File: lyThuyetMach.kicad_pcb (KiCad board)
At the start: 2 copper layers, 48 x 79 mm, 34 parts, among them J1 USB_C_Receptacle_PowerOnly_6P, J2 Voltage_Booster, J4 Out_LED, Q1 BC547, Q2 BC547, Q3 BC547, Q4 BC547, Q5 BC547, Q6 BC547, Q7 TIP122, SW1 SW_SPDT, SW2 SW_SPDT

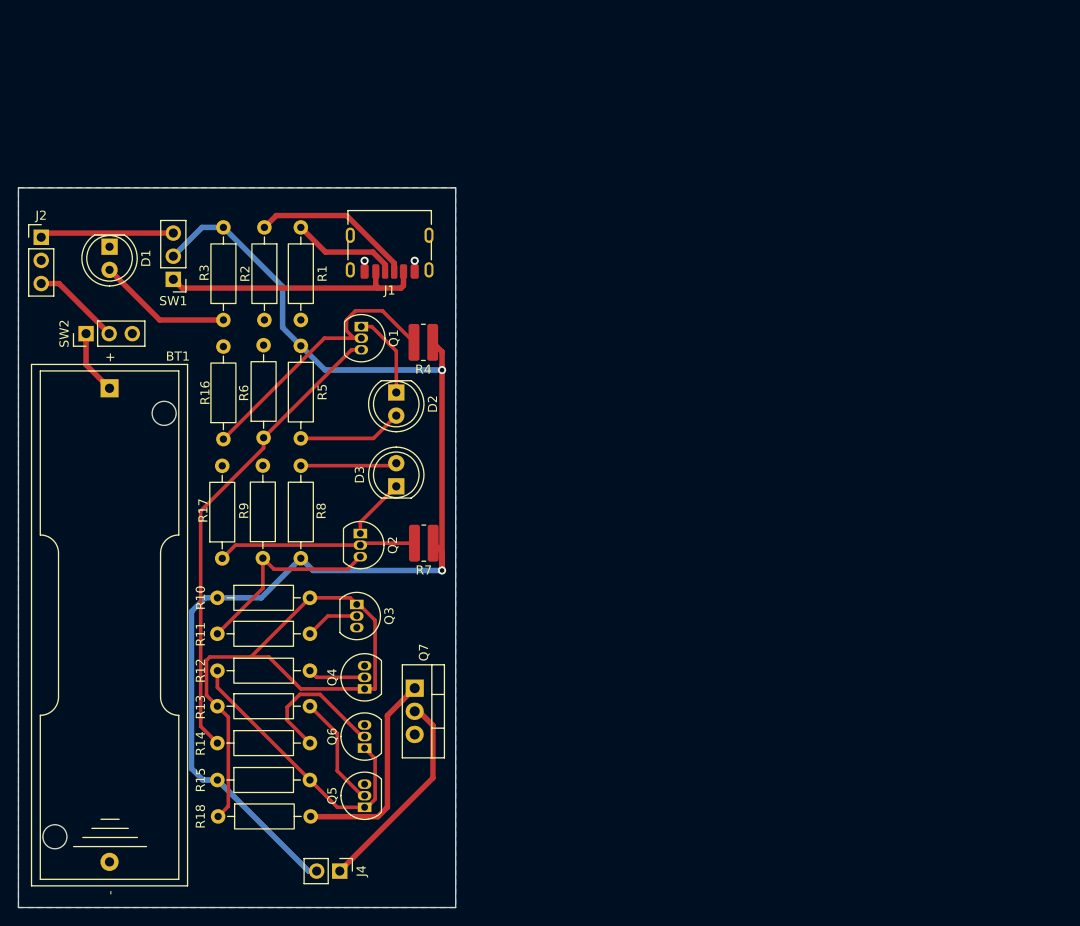
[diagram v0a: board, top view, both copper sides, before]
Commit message: Add files via upload
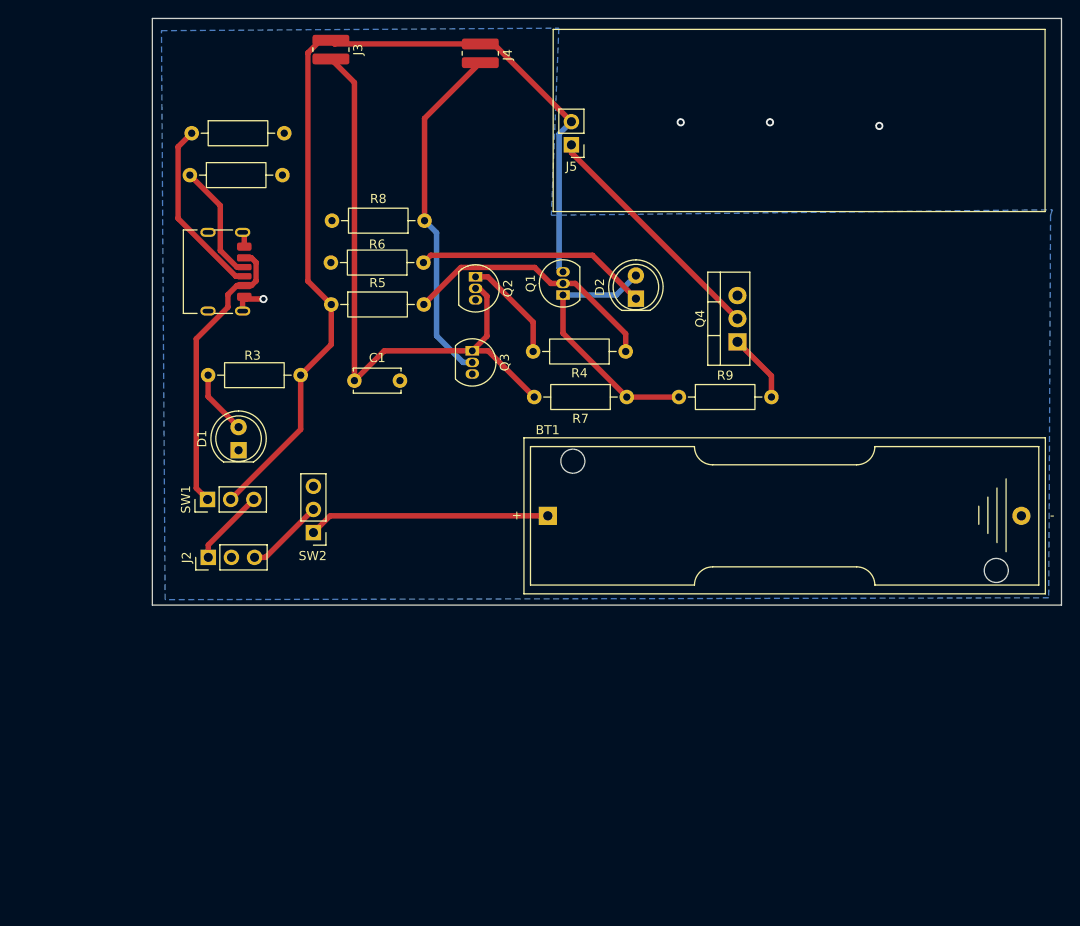
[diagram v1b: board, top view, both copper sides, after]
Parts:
- removed D3: LED, LED_THT:LED_D5.0mm_FlatTop
- removed Q5, Q6: BC547, Package_TO_SOT_THT:TO-92_Inline
- removed Q7: TIP122, Package_TO_SOT_THT:TO-220-3_Vertical
- removed R10, R15: 470, Resistor_THT:R_Axial_DIN0207_L6.3mm_D2.5mm_P10.16mm_Horizontal
- removed R11, R12, R13, R14, R18: 1k, Resistor_THT:R_Axial_DIN0207_L6.3mm_D2.5mm_P10.16mm_Horizontal
- removed R16, R17: 1M, Resistor_THT:R_Axial_DIN0207_L6.3mm_D2.5mm_P10.16mm_Horizontal
- added C1: 100n, Capacitor_THT:C_Disc_D5.0mm_W2.5mm_P5.00mm, F.Cu at (91.4, 66.2)
- added J3: Conn_01x02_Pin, Resistor_SMD:R_0815_2038Metric_Pad1.20x4.05mm_HandSolder, F.Cu at (88.8, 29.8)
- added J5: Out_LED, Connector_PinHeader_2.54mm:PinHeader_1x02_P2.54mm_Vertical, F.Cu at (115.2, 40.3)
- D2: footprint LED_THT:LED_D5.0mm_FlatTop -> LED_THT:LED_D5.0mm
- J4: value Out_LED -> Conn_01x02_Pin; footprint Connector_PinHeader_2.54mm:PinHeader_1x02_P2.54mm_Vertical -> Resistor_SMD:R_0815_2038Metric_Pad1.20x4.05mm_HandSolder
- Q1: value BC547 -> BC557
- Q4: value BC547 -> TIP122; footprint Package_TO_SOT_THT:TO-92_Inline -> Package_TO_SOT_THT:TO-220-3_Vertical
- R4: value 0 -> 4.7k; footprint Resistor_SMD:R_0815_2038Metric_Pad1.20x4.05mm_HandSolder -> Resistor_THT:R_Axial_DIN0207_L6.3mm_D2.5mm_P10.16mm_Horizontal
- R5: value 100 -> 4.7k
- R6, R9: value 4.7k -> 1k
- R7: value 0 -> 10k; footprint Resistor_SMD:R_0815_2038Metric_Pad1.20x4.05mm_HandSolder -> Resistor_THT:R_Axial_DIN0207_L6.3mm_D2.5mm_P10.16mm_Horizontal
- R8: value 100 -> 1M
- moved J4 91.1 mm to (105.2, 30.2)
- moved Q4 55.9 mm to (133.4, 61.9)
- moved BT1 50.1 mm to (112.6, 81.0), turned to 0 degrees
- moved R9 49.0 mm to (127.0, 68.0), turned to 0 degrees
- moved J2 39.6 mm to (75.3, 85.6), turned to 90 degrees
- moved R8 39.5 mm to (99.1, 48.6), turned to 180 degrees
- moved SW2 33.2 mm to (86.9, 82.8), turned to 180 degrees
- moved Q2 30.9 mm to (104.7, 54.8)
- moved Q3 30.6 mm to (104.3, 62.9)
- moved D2 28.2 mm to (122.3, 57.2), turned to 90 degrees
- moved R7 27.5 mm to (121.3, 68.0)
- moved D1 26.5 mm to (78.7, 73.8), turned to 90 degrees
- moved R6 26.0 mm to (99.0, 53.2), turned to 180 degrees
- moved SW1 24.5 mm to (75.3, 79.2), turned to 90 degrees
- moved Q1 22.4 mm to (114.3, 56.8), turned to 90 degrees
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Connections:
- D2 pad 2: Net-(D2-A) -> /LED TOGGLE
- J4 pad 1: Net-(J4-Pin_1) -> VCC
- J4 pad 2: VCC -> Net-(J4-Pin_2)
- Q1 pad 1: Net-(D2-K) -> /LED TOGGLE
- Q1 pad 3: SET -> VCC
- Q2 pad 1: Net-(D3-K) -> Net-(Q2-C)
- Q2 pad 2: Net-(Q2-B) -> Net-(J3-Pin_2)
- Q2 pad 3: RESET -> USB_GND
- Q3 pad 1: LED_Toggle -> Net-(J3-Pin_2)
- Q3 pad 2: Net-(Q3-B) -> Net-(J4-Pin_2)
- Q4 pad 1: LED_Toggle -> Net-(Q4-B)
- Q4 pad 2: Net-(Q4-B) -> /OUT_LED_NE
- R4 pad 1: VCC -> Net-(Q1-B)
- R4 pad 2: Net-(Q1-B) -> Net-(Q2-C)
- R5 pad 2: Net-(D2-A) -> Net-(Q1-B)
- R6 pad 1: SET -> Net-(D2-K)
- R7 pad 1: VCC -> /LED TOGGLE
- R7 pad 2: Net-(Q2-B) -> Net-(J3-Pin_2)
- R8 pad 1: VCC -> Net-(J4-Pin_2)
- R8 pad 2: Net-(D3-A) -> USB_GND
- R9 pad 1: RESET -> /LED TOGGLE
- R9 pad 2: USB_GND -> Net-(Q4-B)
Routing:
- net Net-(J3-Pin_2): track 0.00 -> 68.3 mm
- net LED_Toggle: track 63.6 -> 0.00 mm
- net SET: track 51.9 -> 0.00 mm
- net Net-(J4-Pin_2): track 0.00 -> 38.0 mm
- net NOT_LED_Toggle: track 31.1 -> 0.00 mm
- net VCC: track 135.4 -> 105.1 mm, vias 2 -> 0
- net /LED TOGGLE: track 0.00 -> 28.7 mm
- net /OUT_LED_NE: track 0.00 -> 26.6 mm
- net Net-(Q7-B): track 23.2 -> 0.00 mm
- net Net-(J4-Pin_1): track 22.9 -> 0.00 mm
- net RESET: track 22.1 -> 0.00 mm
- net Net-(Q2-B): track 21.8 -> 0.00 mm
- net Net-(BT1-+): track 7.07 -> 26.7 mm
- net Net-(D2-K): track 9.49 -> 25.6 mm
- net Net-(Q6-B): track 16.0 -> 0.00 mm
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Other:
- board size 48 x 79 mm -> 99.8 x 64.4 mm
